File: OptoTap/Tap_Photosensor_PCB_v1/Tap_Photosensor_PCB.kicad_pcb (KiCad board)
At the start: 2 copper layers, 28.8 x 10.2 mm, 11 parts, among them J1 Conn_01x01_Male, J2 Conn_01x01_Male, J3 Conn_01x01_Male, U1 OPB961N51

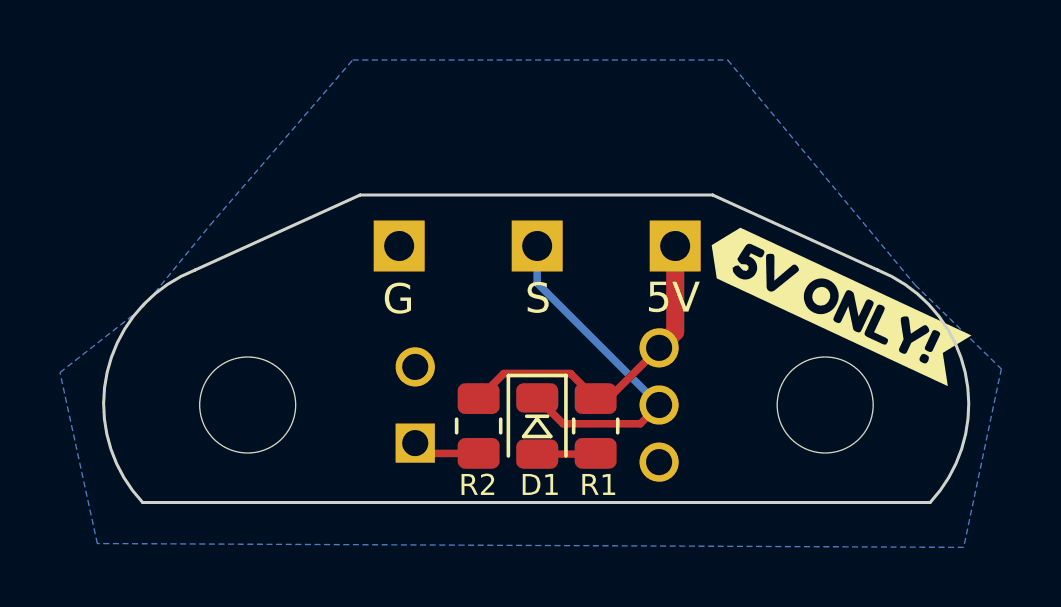
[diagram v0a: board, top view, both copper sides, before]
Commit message: updated OptoTap boards
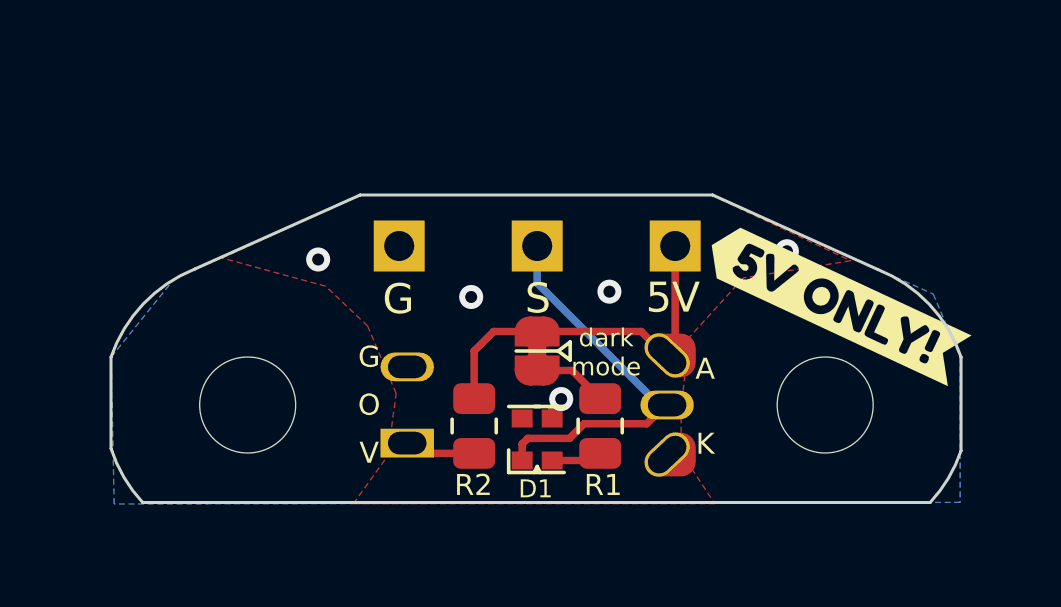
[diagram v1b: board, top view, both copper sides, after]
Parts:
- added JP1: SolderJumper_2_Bridged, Jumper:SolderJumper-2_P1.3mm_Bridged_RoundedPad1.0x1.5mm, F.Cu at (112.4, 63.7)
- D1: value LED -> XL-1615RGBC; footprint LED_SMD:LED_0805_2012Metric -> LED_SMD:LED_0606_1432
- U1: value OPB961N51 -> OPB961N5/EE-SX398; footprint footprints:OPTO_OPB961N51 -> footprints:OPTO_EE-SX398_OPB666N
- moved D1 0.45 mm to (112.4, 66.7), turned to 90 degrees
- moved R1 0.15 mm to (114.5, 66.2)
- moved R2 0.15 mm to (110.3, 66.2)
- turned U1 to 180 degrees
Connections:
- R1 pad 1: +5V -> Net-(JP1-Pad1)
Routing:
- net Net-(JP1-Pad1): track 0.00 -> 2.49 mm
- net +5V: track 11.0 -> 12.5 mm
- net SIG: track 11.7 -> 12.8 mm
- net GND: track 0.00 -> 0.77 mm, vias 0 -> 5
- added copper zone on F.Cu, net GND
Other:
- board size 28.8 x 10.2 mm -> 28.3 x 10.2 mm
- board text added: "dark mode"
- board text added: "rev 1.3"
- board text removed: "OPB666N OPB971"
- board text removed: "rev 1.0"
